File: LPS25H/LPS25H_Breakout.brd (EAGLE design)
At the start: 15.2 x 11.2 mm, 2 parts

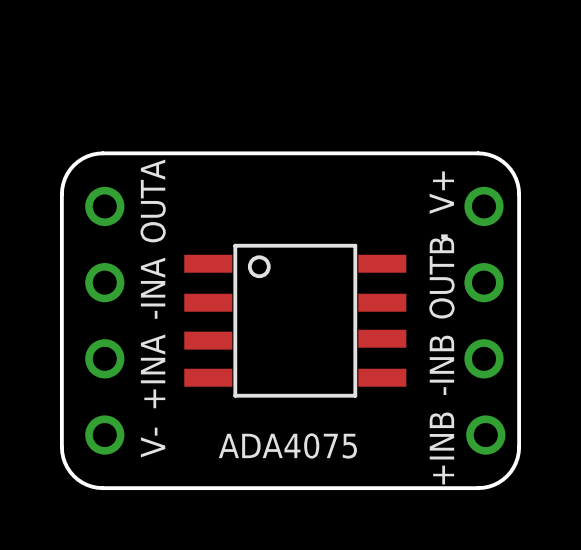
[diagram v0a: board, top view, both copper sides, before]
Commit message: Update new meme.
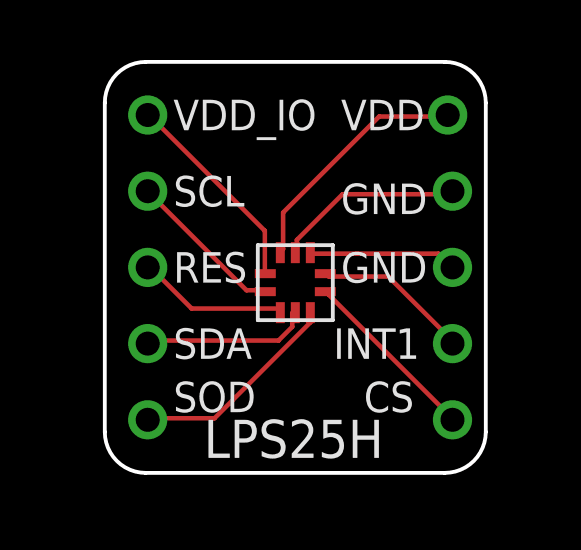
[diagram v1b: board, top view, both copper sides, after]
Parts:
- removed .: ADA4075, FaBo-Opamp:SOIC(NARROW)-8
- removed U$3: 8PIN, FaBo-Breakout:8PIN
- added U$1: ST-LPS25H, FaBo-Mems:ST-LPS25H
- added U$2: 10PIN, FaBo-Breakout:10PIN
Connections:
- removed net 1: ..1, U$3.1
- removed net 2: ..2, U$3.2
- removed net 3: ..3, U$3.3
- removed net 4: ..4, U$3.4
- removed net 5: ..5, U$3.5
- removed net 6: ..6, U$3.6
- removed net 7: ..7, U$3.7
- removed net 8: ..8, U$3.8
- new net CS: U$1.6, U$2.6
- new net GND@8: U$1.8, U$2.8
- new net GND@9: U$1.9, U$2.9
- new net INT1: U$1.7, U$2.7
- new net RES: U$1.3, U$2.3
- new net SCL: U$1.2, U$2.2
- new net SDA: U$1.4, U$2.4
- new net SDO: U$1.5, U$2.5
- new net VDD: U$1.10, U$2.10
- new net VDD_IO: U$1.1, U$2.1
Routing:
- net VDD: track 0.00 -> 8.23 mm
- net SDO: track 0.00 -> 7.09 mm
- net VDD_IO: track 0.00 -> 6.92 mm
- net GND@9: track 0.00 -> 6.35 mm
- net CS: track 0.00 -> 6.03 mm
- net SDA: track 0.00 -> 5.61 mm
- net SCL: track 0.00 -> 5.32 mm
- net INT1: track 0.00 -> 5.25 mm
- net RES: track 0.00 -> 5.08 mm
- net GND@8: track 0.00 -> 4.96 mm
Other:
- board size 15.2 x 11.2 mm -> 12.7 x 13.7 mm
- board text added: "CS"
- board text added: "GND"
- board text added: "INT1"
- board text added: "LPS25H"
- board text added: "RES"
- board text added: "SCL"
- board text added: "SDA"
- board text added: "SOD"
- board text added: "VDD"
- board text added: "VDD_IO"
- board text removed: "+INA"
- board text removed: "+INB"
- board text removed: "-INA"
- board text removed: "-INB"
- board text removed: "ADA4075"
- board text removed: "OUTA"
- board text removed: "OUTB"
- board text removed: "V+"
- board text removed: "V-"
